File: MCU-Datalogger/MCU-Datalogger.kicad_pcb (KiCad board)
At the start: 2 copper layers, 51.3 x 34 mm, 29 parts, among them J1 Conn_01x04_Pin, J2 Conn_01x04_Pin, J3 Conn_01x09_Pin, J4 Conn_02x03_Odd_Even, U1 24LC1025, U2 24LC1025, U3 DS1337S+, U4 ATMEGA328P-AU, Y1 32.768 KHz, Y2 16 MHz

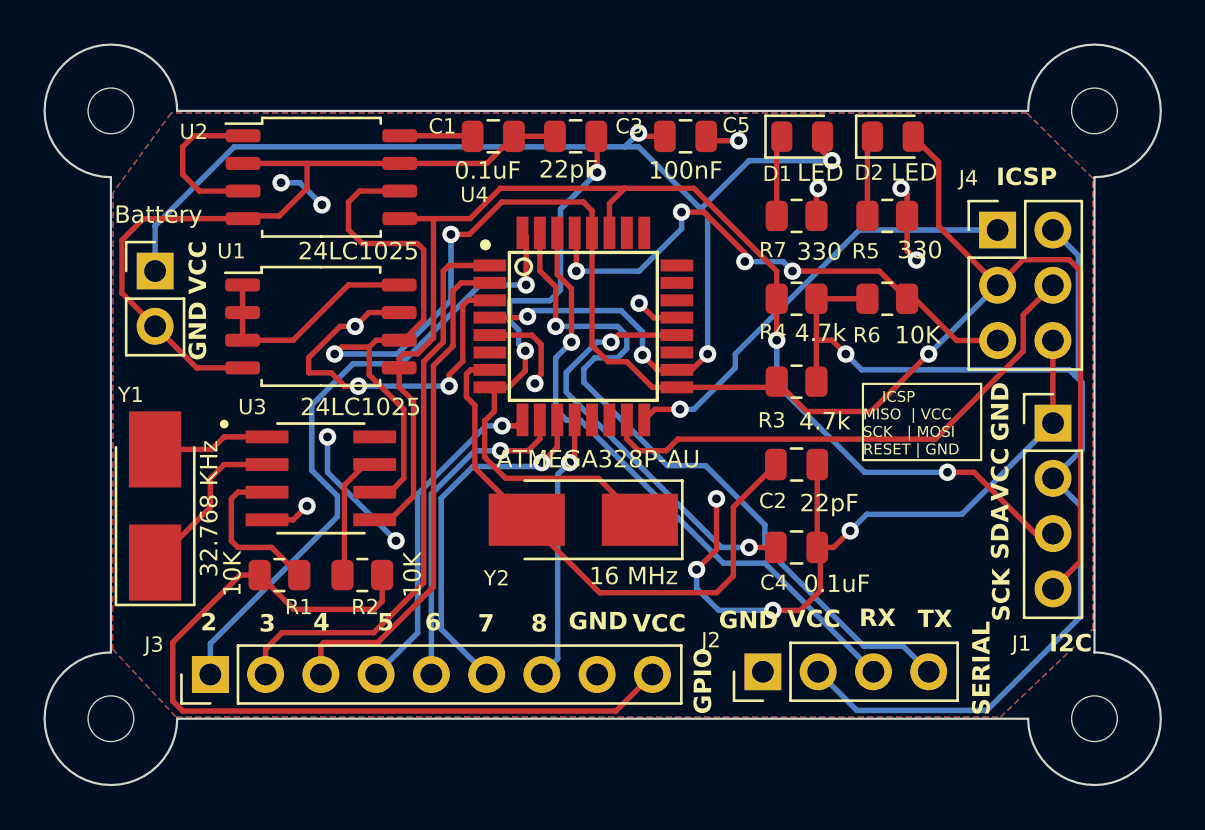
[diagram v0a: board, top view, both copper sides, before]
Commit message: complet 2Layer pcb
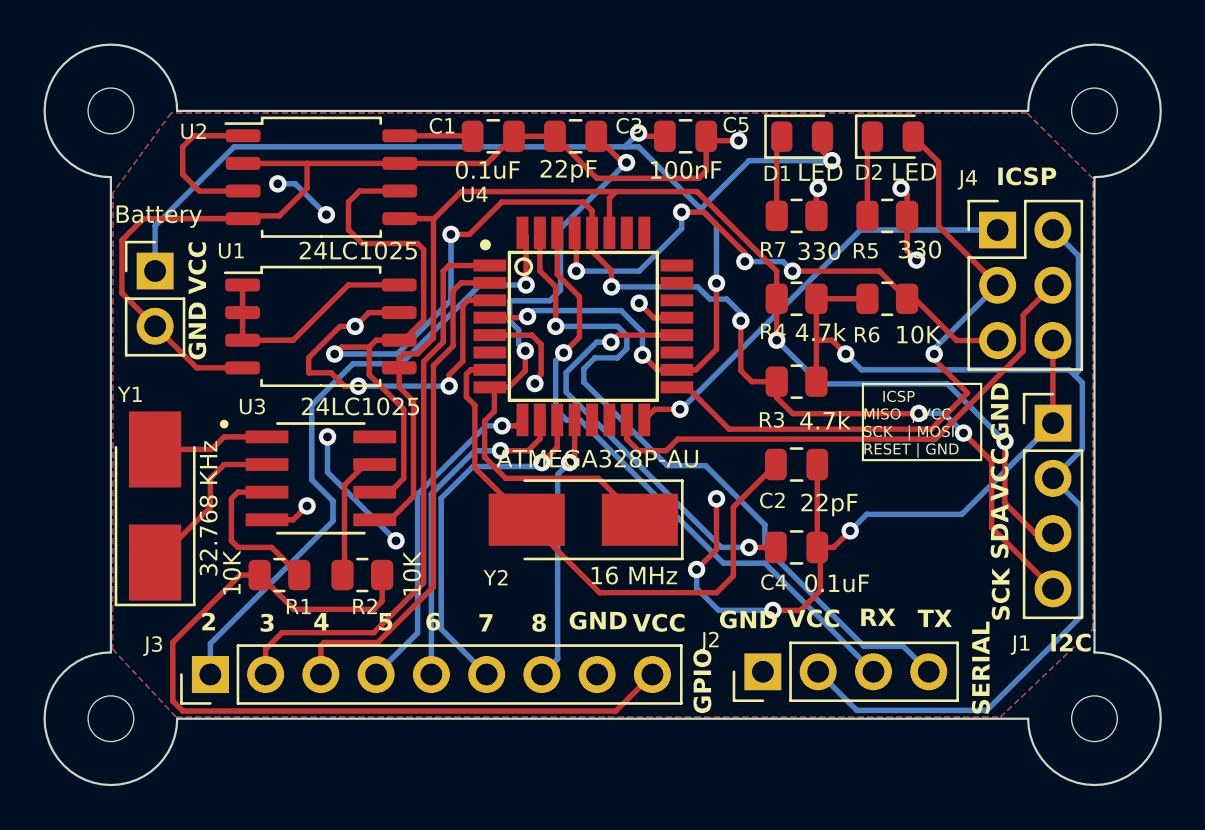
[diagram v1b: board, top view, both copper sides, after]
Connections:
- J1 pad 4: /SCK -> /SCL
- R3 pad 2: /SCK -> /SCL
- U1 pad 6: /SCK -> /SCL
- U2 pad 6: /SCK -> /SCL
- U3 pad 6: /SCK -> /SCL
- U4 pad 28: /SCK -> /SCL
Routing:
- net /SCL: track 0.00 -> 74.3 mm, vias 0 -> 6
- net /SCK: track 97.4 -> 30.1 mm, vias 3 -> 1
- net GND: track 101.7 -> 111.2 mm
- net Net-(U4-PB7): track 27.6 -> 28.8 mm
- net /Vcc: track 181.1 -> 182.0 mm
